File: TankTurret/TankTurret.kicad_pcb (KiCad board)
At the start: 2 copper layers, 35 x 60 mm, 65 parts, among them J1 Conn_01x04_Socket, J2 USB_C_Receptacle_USB2.0_16P, J4 Conn_01x02, J5 Conn_01x02, J6 Conn_01x03, Q1 MMBT3904, SW1 SW_Push, SW2 SW_Push, U1 ESP32-S3-WROOM-1, U3 ME6211C28M5G, U4 LN1234B132MR-G

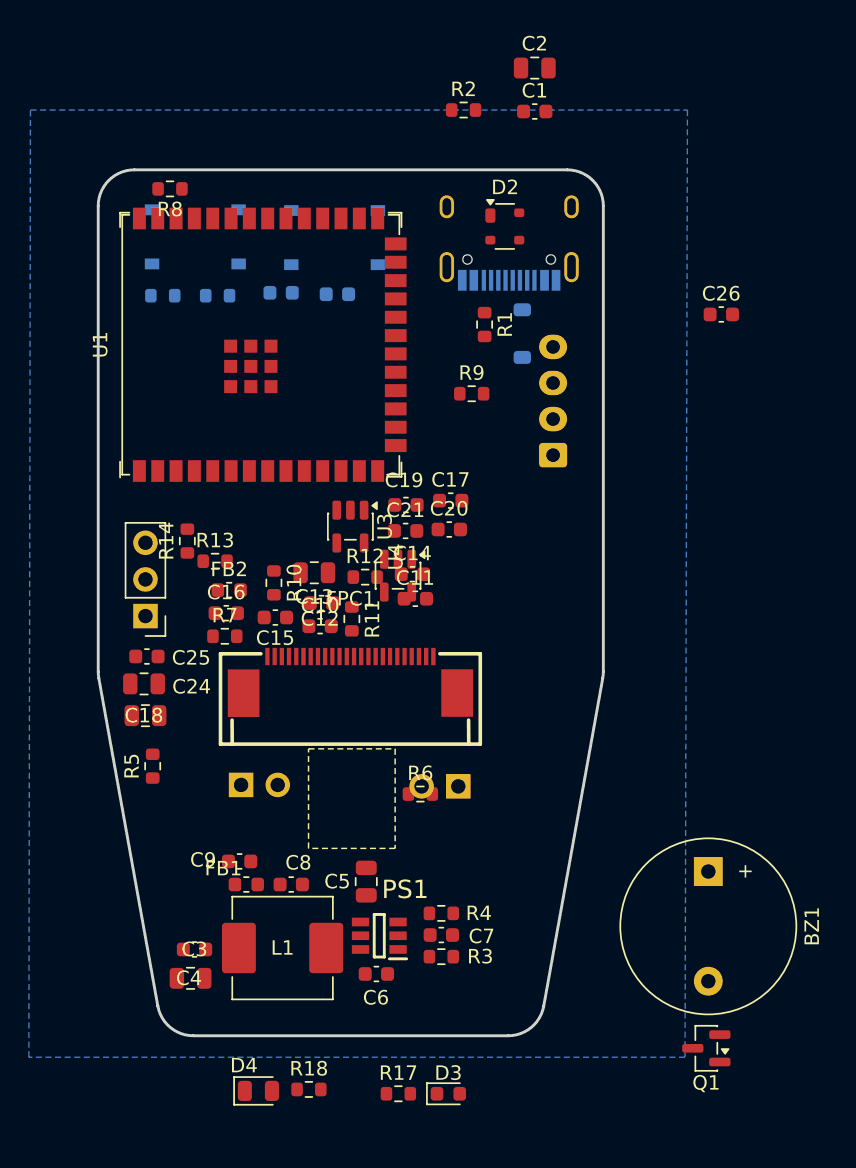
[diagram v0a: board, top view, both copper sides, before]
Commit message: Signed-off-by: SMAUG\Pete <pwbrophy@gmail.com>
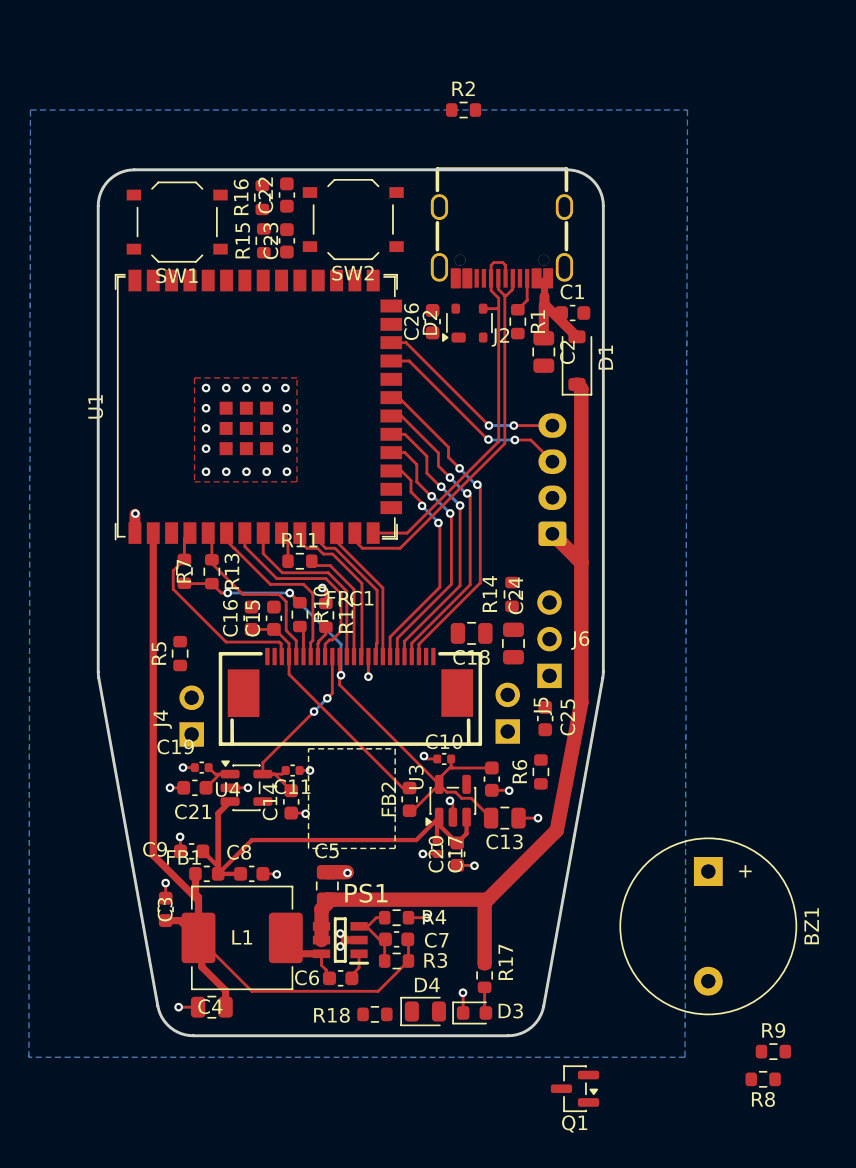
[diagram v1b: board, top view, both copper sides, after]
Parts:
- C10, C11, C17, C19: footprint Capacitor_SMD:C_0603_1608Metric -> Capacitor_SMD:C_0402_1005Metric
- C22, C23, D1, R15, R16, SW1, SW2: moved to F.Cu
- J2: footprint Connector_USB:USB_C_Receptacle_HRO_TYPE-C-31-M-12 -> EasyEDA2Kicad:USB-C_SMD-TYPE-C-31-M-12_1; moved to F.Cu
- J6: moved to B.Cu
- moved R8 74.1 mm to (99.9, 104.3)
- moved R9 50.1 mm to (100.6, 102.4)
- moved J6 28.3 mm to (85.1, 76.3), turned to 0 degrees
- moved C25 27.9 mm to (84.8, 79.3), turned to 90 degrees
- moved C24 25.8 mm to (82.6, 74.1), turned to 90 degrees
- moved C17 24.0 mm to (77.3, 88.2), turned to 90 degrees
- moved C18 23.3 mm to (79.7, 73.4)
- moved C19 23.1 mm to (61.0, 82.7)
- moved C21 23.0 mm to (60.5, 84.1)
- moved R14 22.8 mm to (82.5, 70.7)
- moved C20 22.5 mm to (78.7, 88.7), turned to 90 degrees
- moved C13 21.5 mm to (82.0, 86.2)
- moved U3 20.3 mm to (78.4, 85.0), turned to 90 degrees
- moved C26 20.0 mm to (77.0, 51.8), turned to 90 degrees
- moved C2 19.7 mm to (84.7, 53.9), turned to -90 degrees
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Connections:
- FPC1 pad 12: /GPIO16 -> /GPIO15
- FPC1 pad 17: /GPIO13 -> /GPIO8
- FPC1 pad 18: /GPIO12 -> /GPIO9
- FPC1 pad 19: /GPIO11 -> /GPIO10
- FPC1 pad 20: /GPIO10 -> /GPIO11
- FPC1 pad 21: /GPIO9 -> /GPIO12
- FPC1 pad 22: /GPIO8 -> /GPIO13
- R1 pad 1: Net-(J2-CC1) -> Net-(J2-CC2)
- R11 pad 1: /GPIO15 -> /GPIO16
- R2 pad 1: Net-(J2-CC2) -> Net-(J2-CC1)
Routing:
- net +BATT: track 0.00 -> 59.4 mm
- net +3V3: track 0.00 -> 58.1 mm
- net +CAM_2V8: track 0.00 -> 40.0 mm, vias 0 -> 3
- net +3V3_CLEAN: track 0.00 -> 35.6 mm
- net /USB_D-: track 0.00 -> 27.3 mm
- net /USB_D+: track 0.00 -> 26.9 mm
- net GND: track 0.00 -> 26.4 mm, vias 0 -> 39
- net /GPIO13: track 0.00 -> 22.6 mm, vias 0 -> 2
- net /GPIO12: track 0.00 -> 21.1 mm, vias 0 -> 2
- net /GPIO11: track 0.00 -> 19.6 mm, vias 0 -> 2
- net /GPIO10: track 0.00 -> 18.0 mm, vias 0 -> 2
- net +CAM_AVDD_2V8: track 0.00 -> 16.8 mm
- net /GPIO9: track 0.00 -> 16.3 mm, vias 0 -> 2
- net /GPIO4: track 0.00 -> 14.3 mm
- net +CAM_1V3: track 0.00 -> 14.3 mm, vias 0 -> 2
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- added copper zone on F.Cu, net GND
